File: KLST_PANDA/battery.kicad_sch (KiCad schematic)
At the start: 18 parts, among them Q1 AO3401A, Q2 BCM857BS, SW3 SW_SPST, U7 TP5400

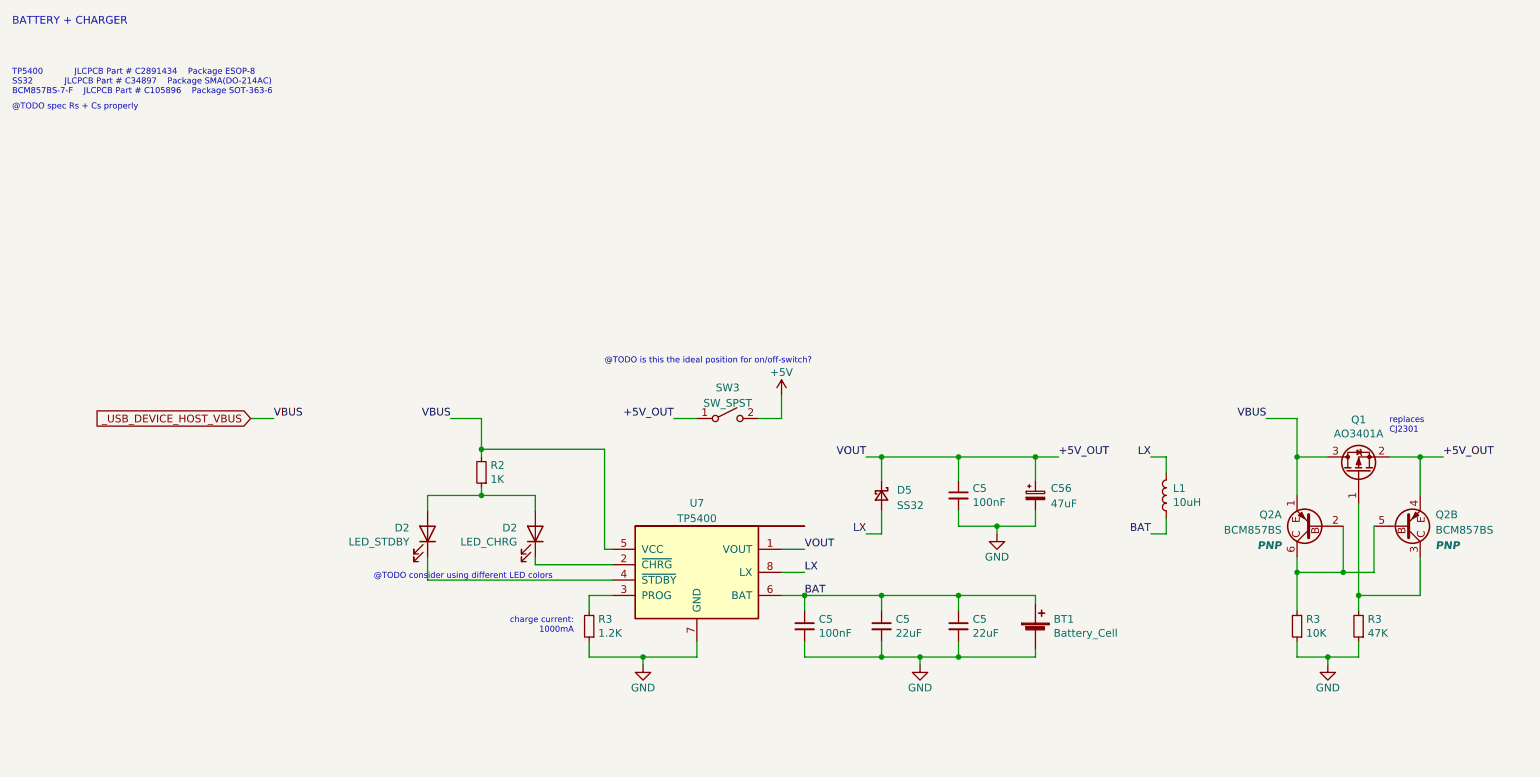
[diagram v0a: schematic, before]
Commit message: cleaned up main sheet
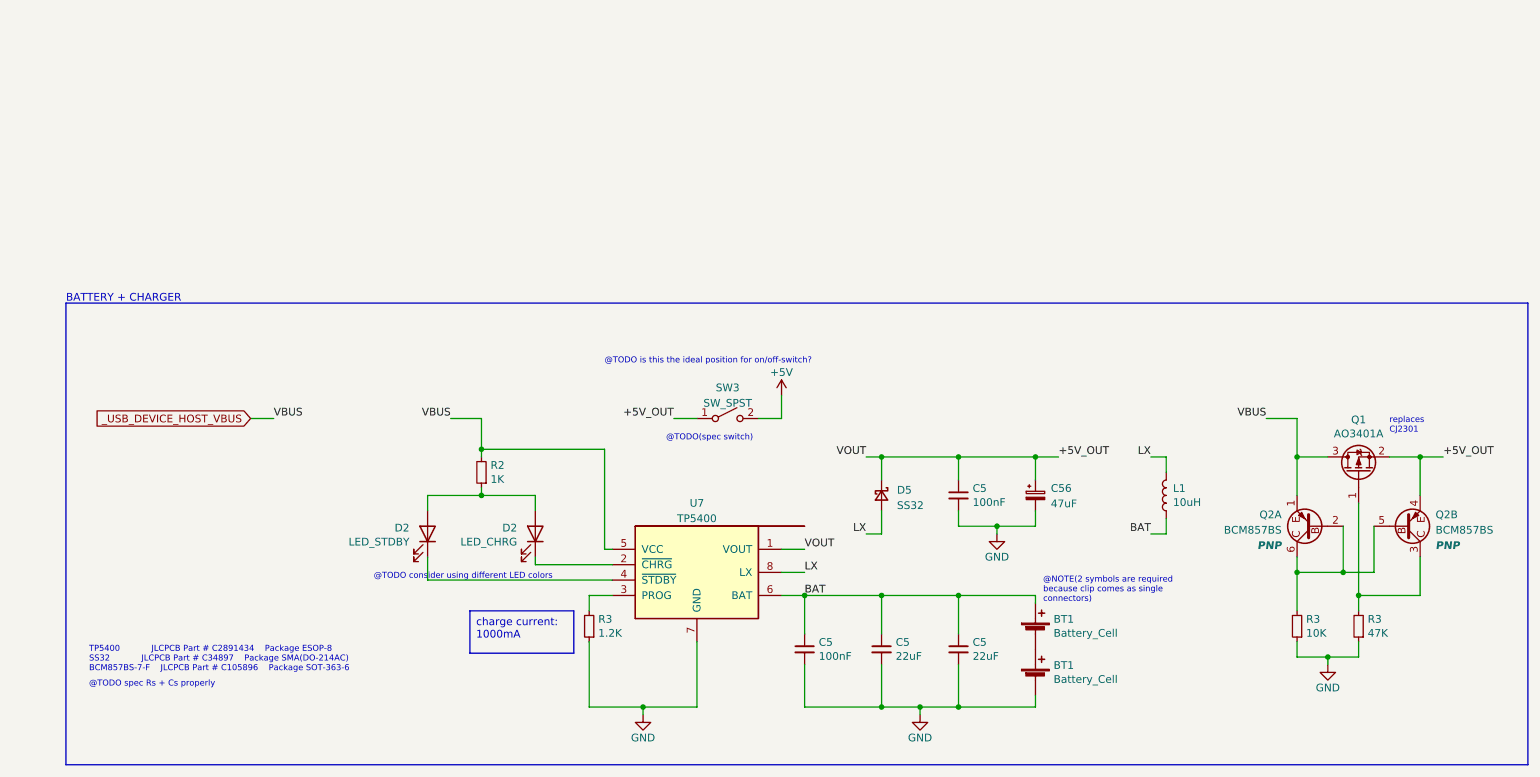
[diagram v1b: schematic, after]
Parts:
- added BT1: Battery_Cell, KLST_GRASS:Keystone Electronics - PC Battery Clip #54, symbol Device:Battery_Cell
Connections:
- net BAT: now also BT1.1 (+); no longer BT1.1 (+)
- new net: BT1.1 (+), BT1.2 (-)
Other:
- note added: "@NOTE(2 symbols are required because clip comes as single connectors)"
- note added: "@TODO(spec switch)"
- note removed: "charge current: 1000mA"
- moved on the sheet: BT1, C5
